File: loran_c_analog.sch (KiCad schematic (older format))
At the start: 62 parts, among them P601 DAC VCO, P602 DAC AGC, P603 QUAD In, P604 LORAN In, Q601 BD135, Q602 BD136, U601 TL072, U602 LD1117S33

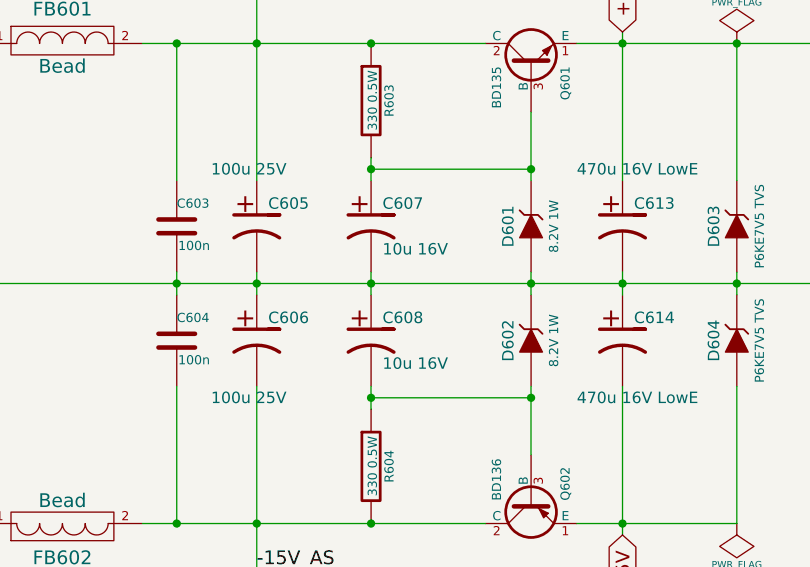
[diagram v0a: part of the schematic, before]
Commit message: Update: PCB routing still in process...
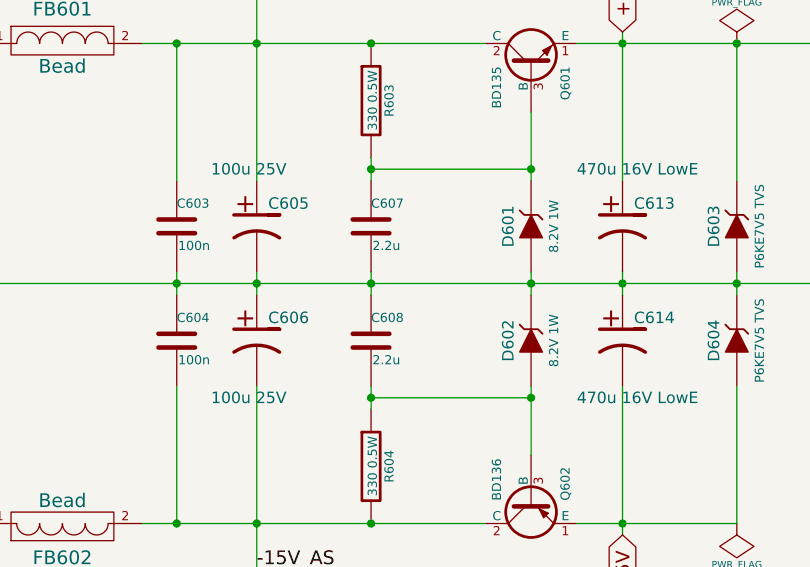
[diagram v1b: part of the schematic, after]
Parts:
- removed C607, C608: 10u 16V, w_pth_capacitors:CP_5x11mm, symbol CP1
- added C607, C608: 2.2u, w_smd_capacitors:c_1206, symbol C
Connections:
- net AGND: now also C607.2, C608.1
- net at D601.2 (K), Q601.3 (B), R603.2: now also C607.1
- net at D602.1 (A), Q602.3 (B), R604.1: now also C608.2
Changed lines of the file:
@@
 LIBS:video
 LIBS:led_holder
+LIBS:crystal_shielded
 LIBS:loran_c_proc_board-cache
 EELAYER 24 0
@@
 $EndComp
 $Comp
-L CP1 C607
-U 1 1 52E34308
-P 3000 2100
-F 0 "C607" H 3050 2200 50  0000 L CNN
-F 1 "10u 16V" H 3050 2000 50  0000 L CNN
-F 2 "w_pth_capacitors:CP_5x11mm" H 3000 2100 60  0001 C CNN
-F 3 "" H 3000 2100 60  0000 C CNN
-	1    3000 2100
-	1    0    0    -1
-$EndComp
-$Comp
 L BD135 Q601
 U 1 1 52E3432C
@@
 $EndComp
 $Comp
-L +3.3VADC #PWR0112
+L +3.3VADC #PWR0109
 U 1 1 52E38762
 P 7700 1650
-F 0 "#PWR0112" H 7700 1770 20  0001 C CNN
+F 0 "#PWR0109" H 7700 1770 20  0001 C CNN
 F 1 "+3.3VADC" H 7700 1740 30  0000 C CNN
 F 2 "" H 7700 1650 60  0000 C CNN
@@
 $EndComp
 $Comp
-L CP1 C608
-U 1 1 52E3AA98
-P 3000 2600
-F 0 "C608" H 3050 2700 50  0000 L CNN
-F 1 "10u 16V" H 3050 2500 50  0000 L CNN
-F 2 "w_pth_capacitors:CP_5x11mm" H 3000 2600 60  0001 C CNN
-F 3 "" H 3000 2600 60  0000 C CNN
-	1    3000 2600
-	1    0    0    -1
-$EndComp
-$Comp
 L ZENER D602
 U 1 1 52E3AADB
@@
 -7.5V
 $Comp
-L AGND #PWR0113
+L AGND #PWR0110
 U 1 1 52E3C710
 P 1150 2400
-F 0 "#PWR0113" H 1150 2400 40  0001 C CNN
+F 0 "#PWR0110" H 1150 2400 40  0001 C CNN
 F 1 "AGND" H 1150 2330 50  0000 C CNN
 F 2 "" H 1150 2400 60  0000 C CNN
@@
 $EndComp
 $Comp
-L AGND #PWR0114
+L AGND #PWR0111
 U 1 1 52E42BA3
 P 3600 4850
-F 0 "#PWR0114" H 3600 4850 40  0001 C CNN
+F 0 "#PWR0111" H 3600 4850 40  0001 C CNN
 F 1 "AGND" H 3600 4780 50  0000 C CNN
 F 2 "" H 3600 4850 60  0000 C CNN
@@
 $EndComp
 $Comp
-L AGND #PWR0115
+L AGND #PWR0112
 U 1 1 52E42BAE
 P 3900 4850
-F 0 "#PWR0115" H 3900 4850 40  0001 C CNN
+F 0 "#PWR0112" H 3900 4850 40  0001 C CNN
 F 1 "AGND" H 3900 4780 50  0000 C CNN
 F 2 "" H 3900 4850 60  0000 C CNN
@@
 $EndComp
 $Comp
-L AGND #PWR0116
+L AGND #PWR0113
 U 1 1 52E434DA
 P 3600 6550
-F 0 "#PWR0116" H 3600 6550 40  0001 C CNN
+F 0 "#PWR0113" H 3600 6550 40  0001 C CNN
 F 1 "AGND" H 3600 6480 50  0000 C CNN
 F 2 "" H 3600 6550 60  0000 C CNN
@@
 $EndComp
 $Comp
-L AGND #PWR0117
+L AGND #PWR0114
 U 1 1 52E434E0
 P 3900 6550
-F 0 "#PWR0117" H 3900 6550 40  0001 C CNN
+F 0 "#PWR0114" H 3900 6550 40  0001 C CNN
 F 1 "AGND" H 3900 6480 50  0000 C CNN
 F 2 "" H 3900 6550 60  0000 C CNN
@@
 $EndComp
 $Comp
-L PWR_FLAG #FLG0118
+L PWR_FLAG #FLG0115
 U 1 1 52E43900
 P 4600 1300
-F 0 "#FLG0118" H 4600 1395 30  0001 C CNN
+F 0 "#FLG0115" H 4600 1395 30  0001 C CNN
 F 1 "PWR_FLAG" H 4600 1480 30  0000 C CNN
 F 2 "" H 4600 1300 60  0000 C CNN
@@
 $EndComp
 $Comp
-L PWR_FLAG #FLG0119
+L PWR_FLAG #FLG0116
 U 1 1 52E4390B
 P 4600 3400
-F 0 "#FLG0119" H 4600 3495 30  0001 C CNN
+F 0 "#FLG0116" H 4600 3495 30  0001 C CNN
 F 1 "PWR_FLAG" H 4600 3580 30  0000 C CNN
 F 2 "" H 4600 3400 60  0000 C CNN
@@
 $EndComp
 $Comp
-L AGND #PWR0120
+L AGND #PWR0117
 U 1 1 52E4434F
 P 4600 5450
-F 0 "#PWR0120" H 4600 5450 40  0001 C CNN
+F 0 "#PWR0117" H 4600 5450 40  0001 C CNN
 F 1 "AGND" H 4600 5380 50  0000 C CNN
 F 2 "" H 4600 5450 60  0000 C CNN
@@
 $EndComp
 $Comp
-L AGND #PWR0121
+L AGND #PWR0118
 U 1 1 52E4435A
 P 4600 6550
-F 0 "#PWR0121" H 4600 6550 40  0001 C CNN
+F 0 "#PWR0118" H 4600 6550 40  0001 C CNN
 F 1 "AGND" H 4600 6480 50  0000 C CNN
 F 2 "" H 4600 6550 60  0000 C CNN
@@
 $EndComp
 $Comp
-L AGND #PWR0122
+L AGND #PWR0119
 U 1 1 52E476C2
 P 1600 5650
-F 0 "#PWR0122" H 1600 5650 40  0001 C CNN
+F 0 "#PWR0119" H 1600 5650 40  0001 C CNN
 F 1 "AGND" H 1600 5580 50  0000 C CNN
 F 2 "" H 1600 5650 60  0000 C CNN
@@
 +-7.5V Opamp voltage regulator
 $Comp
-L AGND #PWR0123
+L AGND #PWR0120
 U 1 1 52E4B7B5
 P 8550 4400
-F 0 "#PWR0123" H 8550 4400 40  0001 C CNN
+F 0 "#PWR0120" H 8550 4400 40  0001 C CNN
 F 1 "AGND" H 8550 4330 50  0000 C CNN
 F 2 "" H 8550 4400 60  0000 C CNN
@@
 $EndComp
 $Comp
-L AGND #PWR0124
+L AGND #PWR0121
 U 1 1 52E4C26B
 P 9050 4100
-F 0 "#PWR0124" H 9050 4100 40  0001 C CNN
+F 0 "#PWR0121" H 9050 4100 40  0001 C CNN
 F 1 "AGND" H 9050 4030 50  0000 C CNN
 F 2 "" H 9050 4100 60  0000 C CNN
@@
 $EndComp
 $Comp
-L AGND #PWR0125
+L AGND #PWR0122
 U 1 1 52E4D87E
 P 8800 4100
-F 0 "#PWR0125" H 8800 4100 40  0001 C CNN
+F 0 "#PWR0122" H 8800 4100 40  0001 C CNN
 F 1 "AGND" H 8800 4030 50  0000 C CNN
 F 2 "" H 8800 4100 60  0000 C CNN
@@
 $EndComp
 $Comp
-L AGND #PWR0126
+L AGND #PWR0123
 U 1 1 52E4EBFE
 P 9700 4100
-F 0 "#PWR0126" H 9700 4100 40  0001 C CNN
+F 0 "#PWR0123" H 9700 4100 40  0001 C CNN
 F 1 "AGND" H 9700 4030 50  0000 C CNN
 F 2 "" H 9700 4100 60  0000 C CNN
@@
 $EndComp
 $Comp
-L AGND #PWR0127
+L AGND #PWR0124
 U 1 1 52E4EC09
 P 10000 4100
-F 0 "#PWR0127" H 10000 4100 40  0001 C CNN
+F 0 "#PWR0124" H 10000 4100 40  0001 C CNN
 F 1 "AGND" H 10000 4030 50  0000 C CNN
 F 2 "" H 10000 4100 60  0000 C CNN
@@
 $EndComp
 $Comp
-L +3.3VADC #PWR0128
+L +3.3VADC #PWR0125
 U 1 1 52E4EC14
 P 9700 2750
-F 0 "#PWR0128" H 9700 2870 20  0001 C CNN
+F 0 "#PWR0125" H 9700 2870 20  0001 C CNN
 F 1 "+3.3VADC" H 9700 2840 30  0000 C CNN
 F 2 "" H 9700 2750 60  0000 C CNN
@@
 $EndComp
 $Comp
-L AGND #PWR0129
+L AGND #PWR0126
 U 1 1 52E53548
 P 10850 4100
-F 0 "#PWR0129" H 10850 4100 40  0001 C CNN
+F 0 "#PWR0126" H 10850 4100 40  0001 C CNN
 F 1 "AGND" H 10850 4030 50  0000 C CNN
 F 2 "" H 10850 4100 60  0000 C CNN
@@
 $EndComp
 $Comp
-L AGND #PWR0130
+L AGND #PWR0127
 U 1 1 52E545D0
 P 9050 5900
-F 0 "#PWR0130" H 9050 5900 40  0001 C CNN
+F 0 "#PWR0127" H 9050 5900 40  0001 C CNN
 F 1 "AGND" H 9050 5830 50  0000 C CNN
 F 2 "" H 9050 5900 60  0000 C CNN
@@
 $EndComp
 $Comp
-L AGND #PWR0131
+L AGND #PWR0128
 U 1 1 52E545EF
 P 8800 5900
-F 0 "#PWR0131" H 8800 5900 40  0001 C CNN
+F 0 "#PWR0128" H 8800 5900 40  0001 C CNN
 F 1 "AGND" H 8800 5830 50  0000 C CNN
 F 2 "" H 8800 5900 60  0000 C CNN
@@
 $EndComp
 $Comp
-L AGND #PWR0132
+L AGND #PWR0129
 U 1 1 52E54601
 P 9700 5900
-F 0 "#PWR0132" H 9700 5900 40  0001 C CNN
+F 0 "#PWR0129" H 9700 5900 40  0001 C CNN
 F 1 "AGND" H 9700 5830 50  0000 C CNN
 F 2 "" H 9700 5900 60  0000 C CNN
@@
 $EndComp
 $Comp
-L AGND #PWR0133
+L AGND #PWR0130
 U 1 1 52E54607
 P 10000 5900
-F 0 "#PWR0133" H 10000 5900 40  0001 C CNN
+F 0 "#PWR0130" H 10000 5900 40  0001 C CNN
 F 1 "AGND" H 10000 5830 50  0000 C CNN
 F 2 "" H 10000 5900 60  0000 C CNN
@@
 $EndComp
 $Comp
-L +3.3VADC #PWR0134
+L +3.3VADC #PWR0131
 U 1 1 52E5460D
 P 9700 4550
-F 0 "#PWR0134" H 9700 4670 20  0001 C CNN
+F 0 "#PWR0131" H 9700 4670 20  0001 C CNN
 F 1 "+3.3VADC" H 9700 4640 30  0000 C CNN
 F 2 "" H 9700 4550 60  0000 C CNN
@@
 $EndComp
 $Comp
-L AGND #PWR0135
+L AGND #PWR0132
 U 1 1 52E54639
 P 10850 5900
-F 0 "#PWR0135" H 10850 5900 40  0001 C CNN
+F 0 "#PWR0132" H 10850 5900 40  0001 C CNN
 F 1 "AGND" H 10850 5830 50  0000 C CNN
 F 2 "" H 10850 5900 60  0000 C CNN
@@
 $EndComp
 $Comp
-L AGND #PWR0136
+L AGND #PWR0133
 U 1 1 52F276DC
 P 8550 2300
-F 0 "#PWR0136" H 8550 2300 40  0001 C CNN
+F 0 "#PWR0133" H 8550 2300 40  0001 C CNN
 F 1 "AGND" H 8550 2230 50  0000 C CNN
 F 2 "" H 8550 2300 60  0000 C CNN
@@
 $EndComp
 $Comp
-L AGND #PWR0137
+L AGND #PWR0134
 U 1 1 52F276E8
 P 9050 2300
-F 0 "#PWR0137" H 9050 2300 40  0001 C CNN
+F 0 "#PWR0134" H 9050 2300 40  0001 C CNN
 F 1 "AGND" H 9050 2230 50  0000 C CNN
 F 2 "" H 9050 2300 60  0000 C CNN
@@
 $EndComp
 $Comp
-L AGND #PWR0138
+L AGND #PWR0135
 U 1 1 52F27707
 P 8800 2300
-F 0 "#PWR0138" H 8800 2300 40  0001 C CNN
+F 0 "#PWR0135" H 8800 2300 40  0001 C CNN
 F 1 "AGND" H 8800 2230 50  0000 C CNN
 F 2 "" H 8800 2300 60  0000 C CNN
@@
 $EndComp
 $Comp
-L AGND #PWR0139
+L AGND #PWR0136
 U 1 1 52F27719
 P 9700 2300
-F 0 "#PWR0139" H 9700 2300 40  0001 C CNN
+F 0 "#PWR0136" H 9700 2300 40  0001 C CNN
 F 1 "AGND" H 9700 2230 50  0000 C CNN
 F 2 "" H 9700 2300 60  0000 C CNN
@@
 $EndComp
 $Comp
-L AGND #PWR0140
+L AGND #PWR0137
 U 1 1 52F2771F
 P 10000 2300
-F 0 "#PWR0140" H 10000 2300 40  0001 C CNN
+F 0 "#PWR0137" H 10000 2300 40  0001 C CNN
 F 1 "AGND" H 10000 2230 50  0000 C CNN
 F 2 "" H 10000 2300 60  0000 C CNN
@@
 $EndComp
 $Comp
-L +3.3VADC #PWR0141
+L +3.3VADC #PWR0138
 U 1 1 52F27725
 P 9700 950
-F 0 "#PWR0141" H 9700 1070 20  0001 C CNN
+F 0 "#PWR0138" H 9700 1070 20  0001 C CNN
 F 1 "+3.3VADC" H 9700 1040 30  0000 C CNN
 F 2 "" H 9700 950 60  0000 C CNN
@@
 $EndComp
 $Comp
-L AGND #PWR0142
+L AGND #PWR0139
 U 1 1 52F27732
 P 10850 2300
-F 0 "#PWR0142" H 10850 2300 40  0001 C CNN
+F 0 "#PWR0139" H 10850 2300 40  0001 C CNN
 F 1 "AGND" H 10850 2230 50  0000 C CNN
 F 2 "" H 10850 2300 60  0000 C CNN
@@
 	8550 4350 8550 4400
 Connection ~ 7800 4350
+$Comp
+L C C607
+U 1 1 53072E90
+P 3000 2100
+F 0 "C607" H 3000 2200 40  0000 L CNN
+F 1 "2.2u" H 3006 2015 40  0000 L CNN
+F 2 "w_smd_capacitors:c_1206" H 3038 1950 30  0001 C CNN
+F 3 "" H 3000 2100 60  0000 C CNN
+	1    3000 2100
+	1    0    0    -1
+$EndComp
+$Comp
+L C C608
+U 1 1 53072EB1
+P 3000 2600
+F 0 "C608" H 3000 2700 40  0000 L CNN
+F 1 "2.2u" H 3006 2515 40  0000 L CNN
+F 2 "w_smd_capacitors:c_1206" H 3038 2450 30  0001 C CNN
+F 3 "" H 3000 2600 60  0000 C CNN
+	1    3000 2600
+	1    0    0    -1
+$EndComp
 $EndSCHEMATC
